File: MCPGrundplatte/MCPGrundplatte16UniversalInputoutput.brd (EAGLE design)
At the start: 49.2 x 80 mm, 60 parts, among them IC2 74HC14N, IC3 74HC14N, IC4 74HC14N, X1GPA0-7 MKDSN1,5/9-5,08, X2GPB0-7 MKDSN1,5/9-5,08

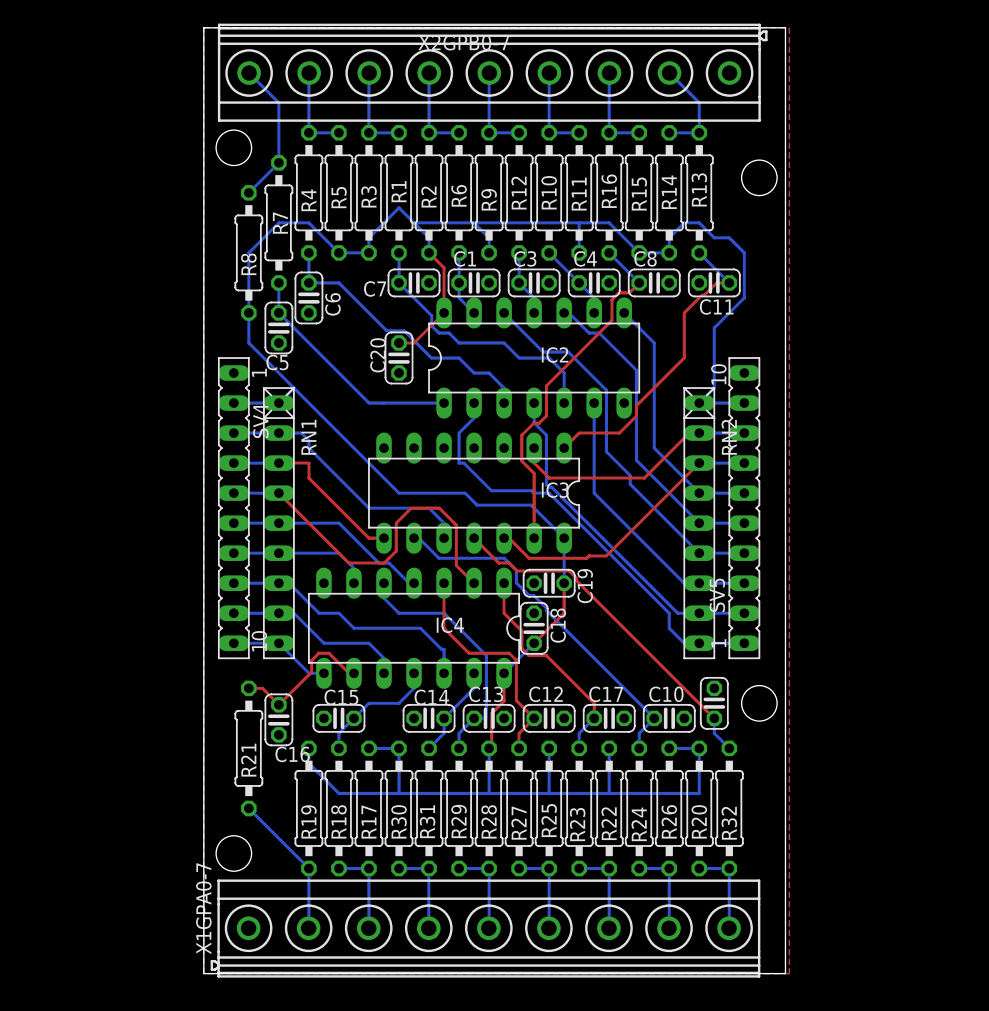
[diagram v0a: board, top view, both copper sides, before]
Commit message: Neu organisiert
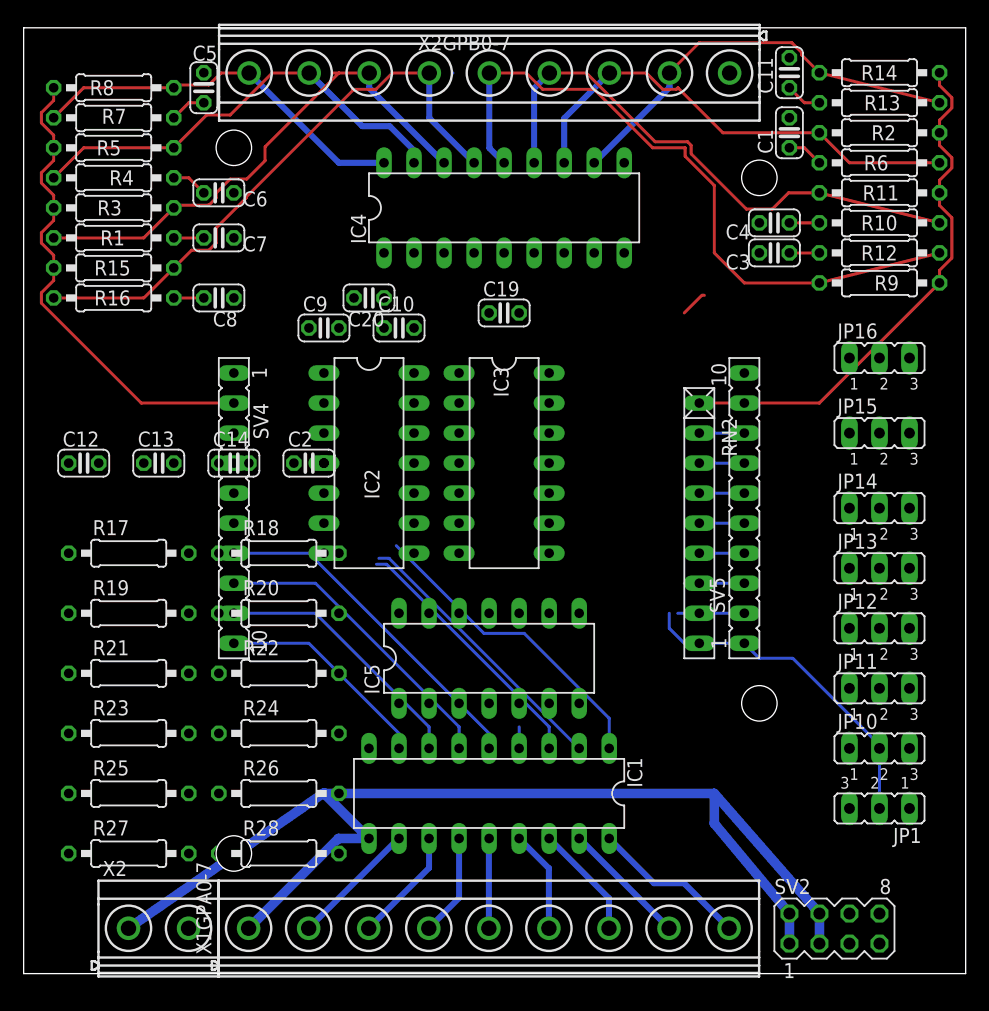
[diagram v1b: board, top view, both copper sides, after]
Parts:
- removed C15, C16, C17, C18, C21: 100nF, rcl:C025-024X044
- removed R29, R30, R31, R32: 10k, rcl:0207/10
- removed RN1: 100K, resistor-net:RN-9
- added C2: 100Nf, rcl:C025-024X044
- added C9: 100nF, rcl:C025-024X044
- added IC1: ULN2803, uln-udn:DIL18
- added IC5: 74HC14N, 74xx-eu:DIL14
- added JP1, JP10, JP11, JP12, JP13, JP14, JP15, JP16: (no value), jumper:JP2
- added SV2: (no value), con-lstb:MA04-2
- added X2: MKDSN1,5/2-5,08, con-phoenix-508:MKDSN1,5/2-5,08
- IC4: value 74HC14N -> ULN2803; device 74xx-eu:DIL14 -> uln-udn:DIL18
- moved C12 44.9 mm to (-10.2, 43.2)
- moved R15 44.9 mm to (-7.62, 59.7), turned to 0 degrees
- moved R16 42.8 mm to (-7.62, 57.1), turned to 0 degrees
- moved C10 40.2 mm to (16.5, 54.6)
- moved R20 39.2 mm to (6.35, 30.5), turned to 0 degrees
- moved R23 38.6 mm to (-6.35, 20.3), turned to 0 degrees
- moved R2 38.4 mm to (57.1, 71.1), turned to 180 degrees
- moved C8 36.9 mm to (1.27, 57.1)
- moved IC4 36.4 mm to (25.4, 64.8), turned to 0 degrees
- moved R6 35.7 mm to (57.1, 68.6), turned to 180 degrees
- moved R25 35.6 mm to (-6.35, 15.2), turned to 0 degrees
- moved C13 35.3 mm to (-3.81, 43.2)
- moved R9 33.9 mm to (57.1, 58.4), turned to 180 degrees
- moved R27 33.2 mm to (-6.35, 10.2), turned to 0 degrees
- moved R26 33.0 mm to (6.35, 15.2), turned to 0 degrees
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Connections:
- removed net GPA0: R20.2, R32.1, X1GPA0-7.9
- removed net GPA1: R24.1, R26.2, X1GPA0-7.8
- removed net GPA2.: IC4.2, RN1.4, SV4.5
- removed net GPA3.: IC4.4, RN1.5, SV4.6
- removed net GPA4.: IC4.6, RN1.6, SV4.7
- removed net GPA5: R30.2, R31.1, X1GPA0-7.4
- removed net GPA6: R17.2, R18.1, X1GPA0-7.3
- removed net GPA7: R19.2, R21.1, X1GPA0-7.2
- removed net GPB7: R13.1, R14.2, X2GPB0-7.2
- removed net N$52: C21.1, IC3.11, R32.2
- new net +12V: IC1.10, IC4.10, SV2.1, SV2.2, SV2.3, SV2.4, X1GPA0-7.1, X2.1
- new net IC2_OUT1: IC1.18, X1GPA0-7.9
- new net IC2_OUT2: IC1.17, X1GPA0-7.8
- new net IC2_OUT3: IC1.16, X1GPA0-7.7
- new net IC2_OUT4: IC1.15, X1GPA0-7.6
- new net IC2_OUT5: IC1.14, X1GPA0-7.5
- new net IC2_OUT6: IC1.13, X1GPA0-7.4
- new net IC2_OUT7: IC1.12, X1GPA0-7.3
- new net IC2_OUT8: IC1.11, X1GPA0-7.2
- new net N$1: IC2.12, JP13.1
- new net N$14: C2.1, IC5.13, R28.2
- new net N$15: IC3.2, JP14.1
- new net N$17: IC4.11, R13.1, R14.2, X2GPB0-7.2
- new net N$18: IC2.6, JP11.1
- new net N$19: IC3.12, JP12.1
- new net N$22: IC4.5, JP15.3
- new net N$23: C13.1, IC5.3, R19.2
- new net N$24: IC4.14, R12.1, R9.2, X2GPB0-7.5
- new net N$25: IC4.6, JP16.3
- new net N$26: IC4.7, JP13.3
- new net N$27: IC4.8, JP14.3
- new net N$29: C12.1, IC5.1, R21.2
- new net N$3: IC2.4, JP10.1
- new net N$30: IC2.2, JP1.1
- new net N$31: C10.1, IC5.9, R23.2
- new net N$32: C9.1, IC5.11, R26.2
- new net N$33: IC4.2, JP10.3
- new net N$34: IC4.1, JP1.3
- new net N$35: R27.2, R28.1
- new net N$37: R21.1, R22.2
- new net N$43: R25.2, R26.1
- net GND: now also C2.2, C9.2, IC1.9, IC3.10, IC3.11, IC3.8, IC3.9, IC4.9, IC5.7, SV2.5, SV2.6, SV2.7, SV2.8, X2.2; no longer C15.2, C16.2, C17.2, C18.1, C21.2, IC4.7, X1GPA0-7.1
- net GPA0.: now also IC1.1; no longer IC3.10, RN1.2
- net GPA1.: now also IC1.2; no longer IC3.8, RN1.3
- net GPA2: now also IC1.3, SV4.5; no longer R22.2, R23.1, X1GPA0-7.7
- net GPA3: now also IC1.4, SV4.6; no longer R25.2, R27.1, X1GPA0-7.6
- net GPA4: now also IC1.5, SV4.7; no longer R28.2, R29.1, X1GPA0-7.5
- net GPA5.: now also IC1.6; no longer IC4.12, RN1.7
- net GPA6.: now also IC1.7; no longer IC4.10, RN1.8
- net GPA7.: now also IC1.8; no longer IC4.8, RN1.9
- net GPB0: now also IC4.18
- net GPB0.: now also JP1.2; no longer IC2.2
- net GPB1: now also IC4.17
- net GPB1.: now also JP10.2; no longer IC2.4
- net GPB2: now also IC4.16
- net GPB2.: now also JP11.2; no longer IC2.6
- net GPB3: now also R17.2, R18.1; no longer R2.2, R6.1, X2GPB0-7.6
- net GPB3.: now also JP12.2; no longer IC2.12
- net GPB4: now also R19.1, R20.1; no longer R12.1, R9.2, X2GPB0-7.5
- net GPB4.: now also JP15.2; no longer IC2.10
- net GPB5: now also IC4.13
- net GPB5.: now also JP16.2; no longer IC2.8
- net GPB6: now also R23.1, R24.2; no longer R15.2, R16.1, X2GPB0-7.3
- net GPB6.: now also JP13.2; no longer IC3.12
- net GPB7.: now also JP14.2; no longer IC3.2
- net N$10: now also IC4.3, JP11.3; no longer C10.1, IC3.9, R24.2
- net N$12: now also IC4.12, R2.2, R6.1, X2GPB0-7.3; no longer C12.1, IC4.3, R27.2
- net N$13: now also IC4.4, JP12.3; no longer C13.1, IC4.5, R29.2
- net N$16: now also C14.1, IC5.5; no longer C15.1, IC4.11
- net N$20: now also IC2.10, JP15.1; no longer C16.1, IC4.9, R21.2
- net N$21: now also IC2.8, JP16.1; no longer C17.1, IC4.1, R23.2
- net N$28: now also IC4.15, R15.2, R16.1, X2GPB0-7.6; no longer C14.1, IC4.13, R31.2
- net VDD: now also IC5.14, R20.2, R24.1; no longer C18.2, IC4.14, R19.1, R20.1, R26.1, R28.1, R30.1, RN1.1
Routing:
- net VDD: track 214.6 -> 85.9 mm
- net +12V: track 0.00 -> 102.9 mm
- net N$24: track 0.00 -> 57.7 mm
- net N$28: track 7.93 -> 49.7 mm
- net GPB5: track 7.60 -> 47.2 mm
- net GPB2: track 7.60 -> 44.2 mm
- net N$17: track 0.00 -> 35.6 mm
- net GPA2.: track 30.7 -> 0.00 mm
- net N$10: track 30.4 -> 0.00 mm
- net GPB1: track 7.60 -> 37.9 mm
- net N$52: track 29.8 -> 0.00 mm
- net GPB3.: track 32.2 -> 3.81 mm
- net N$9: track 30.5 -> 2.54 mm
- net GPB4.: track 27.1 -> 3.81 mm
- net GPB1.: track 28.6 -> 5.63 mm
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- removed copper zone on layer 1, net GND
- removed copper zone on layer 16, net GND
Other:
- board size 49.2 x 80 mm -> 79.7 x 80 mm
